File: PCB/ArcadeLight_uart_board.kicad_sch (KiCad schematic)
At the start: 20 parts, among them J1 Partition_Lights_L, J10 Circle_LED, J11 Cross_LED, J12 Square_LED, J13 Triangle_LED, J3 12V_In, J9 Partition_Lights_R, P7 CONN_01X01, P9 CONN_01X01, Q1 AO3404A, Q2 IRFR9024N, U1 Arduino_Nano_v3.x, U2 ULN2003, U3 ULN2003

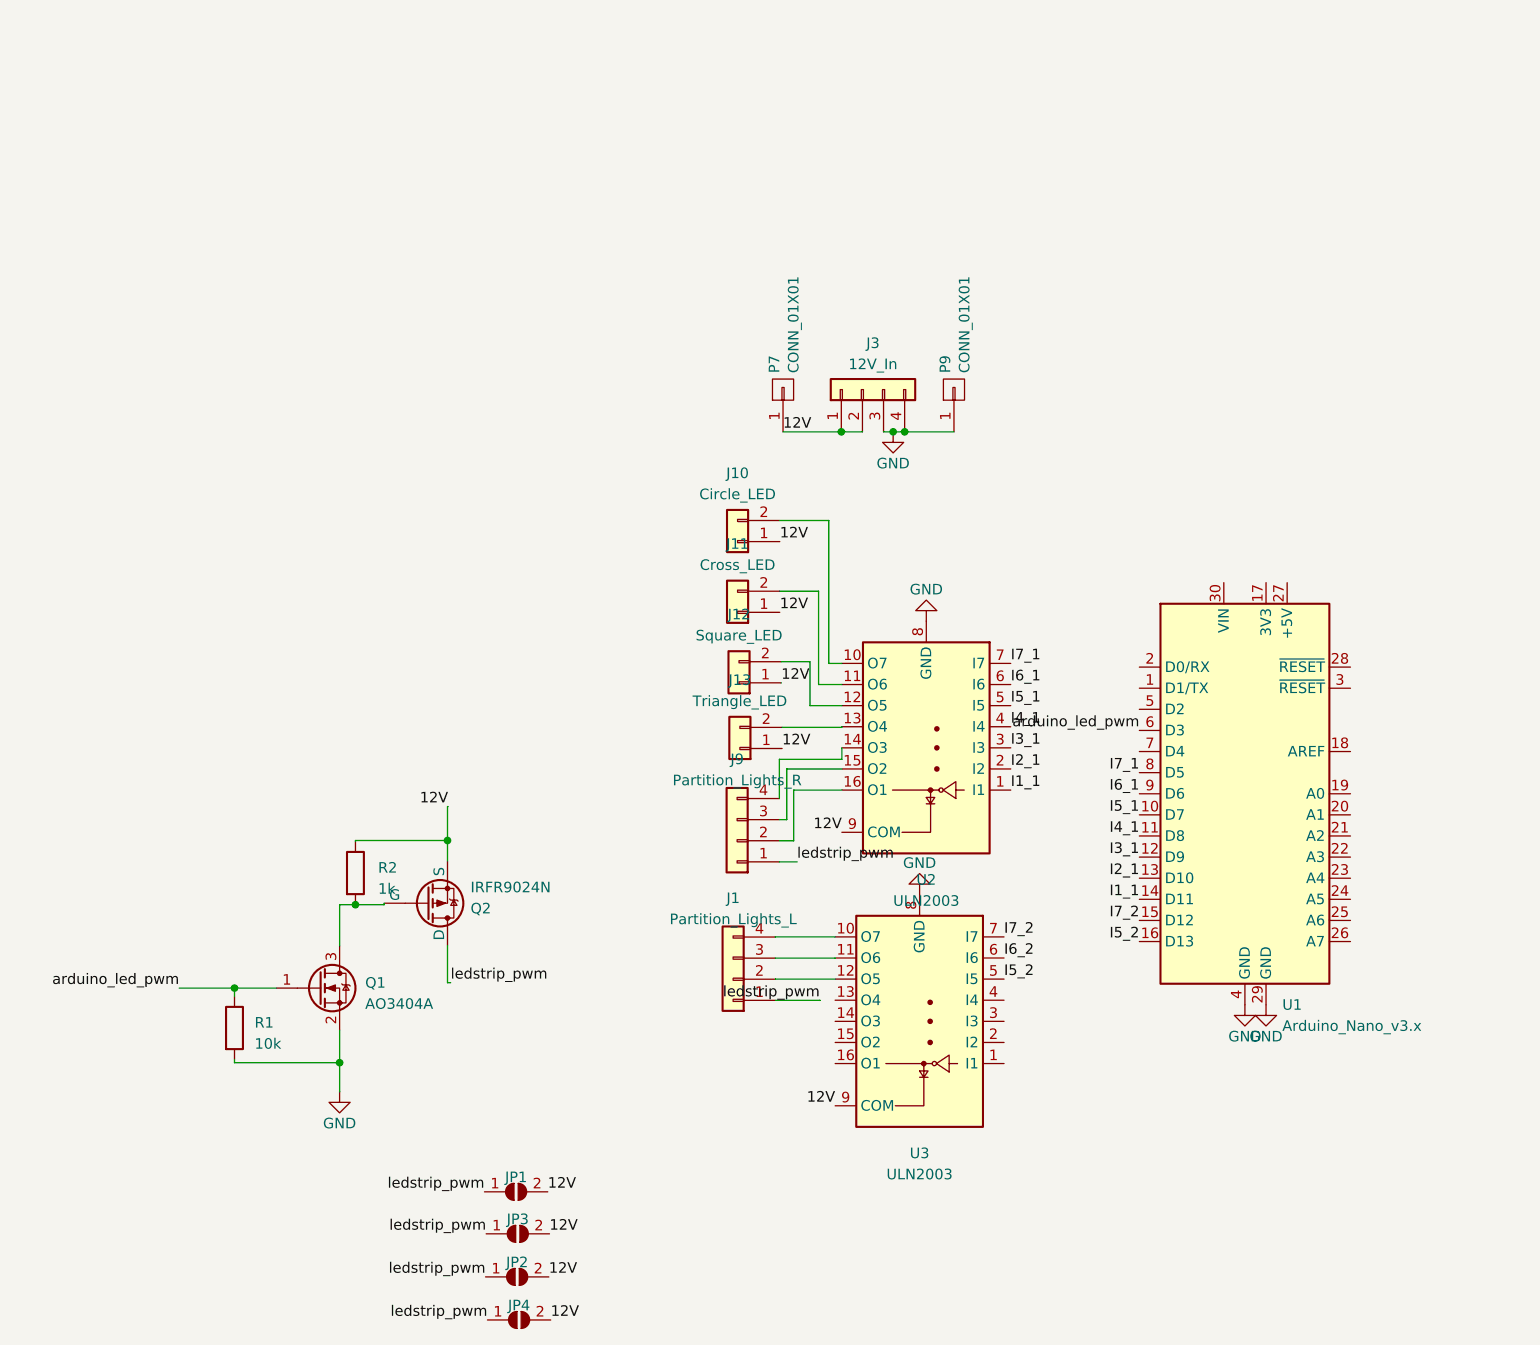
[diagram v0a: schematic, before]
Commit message: Readme update
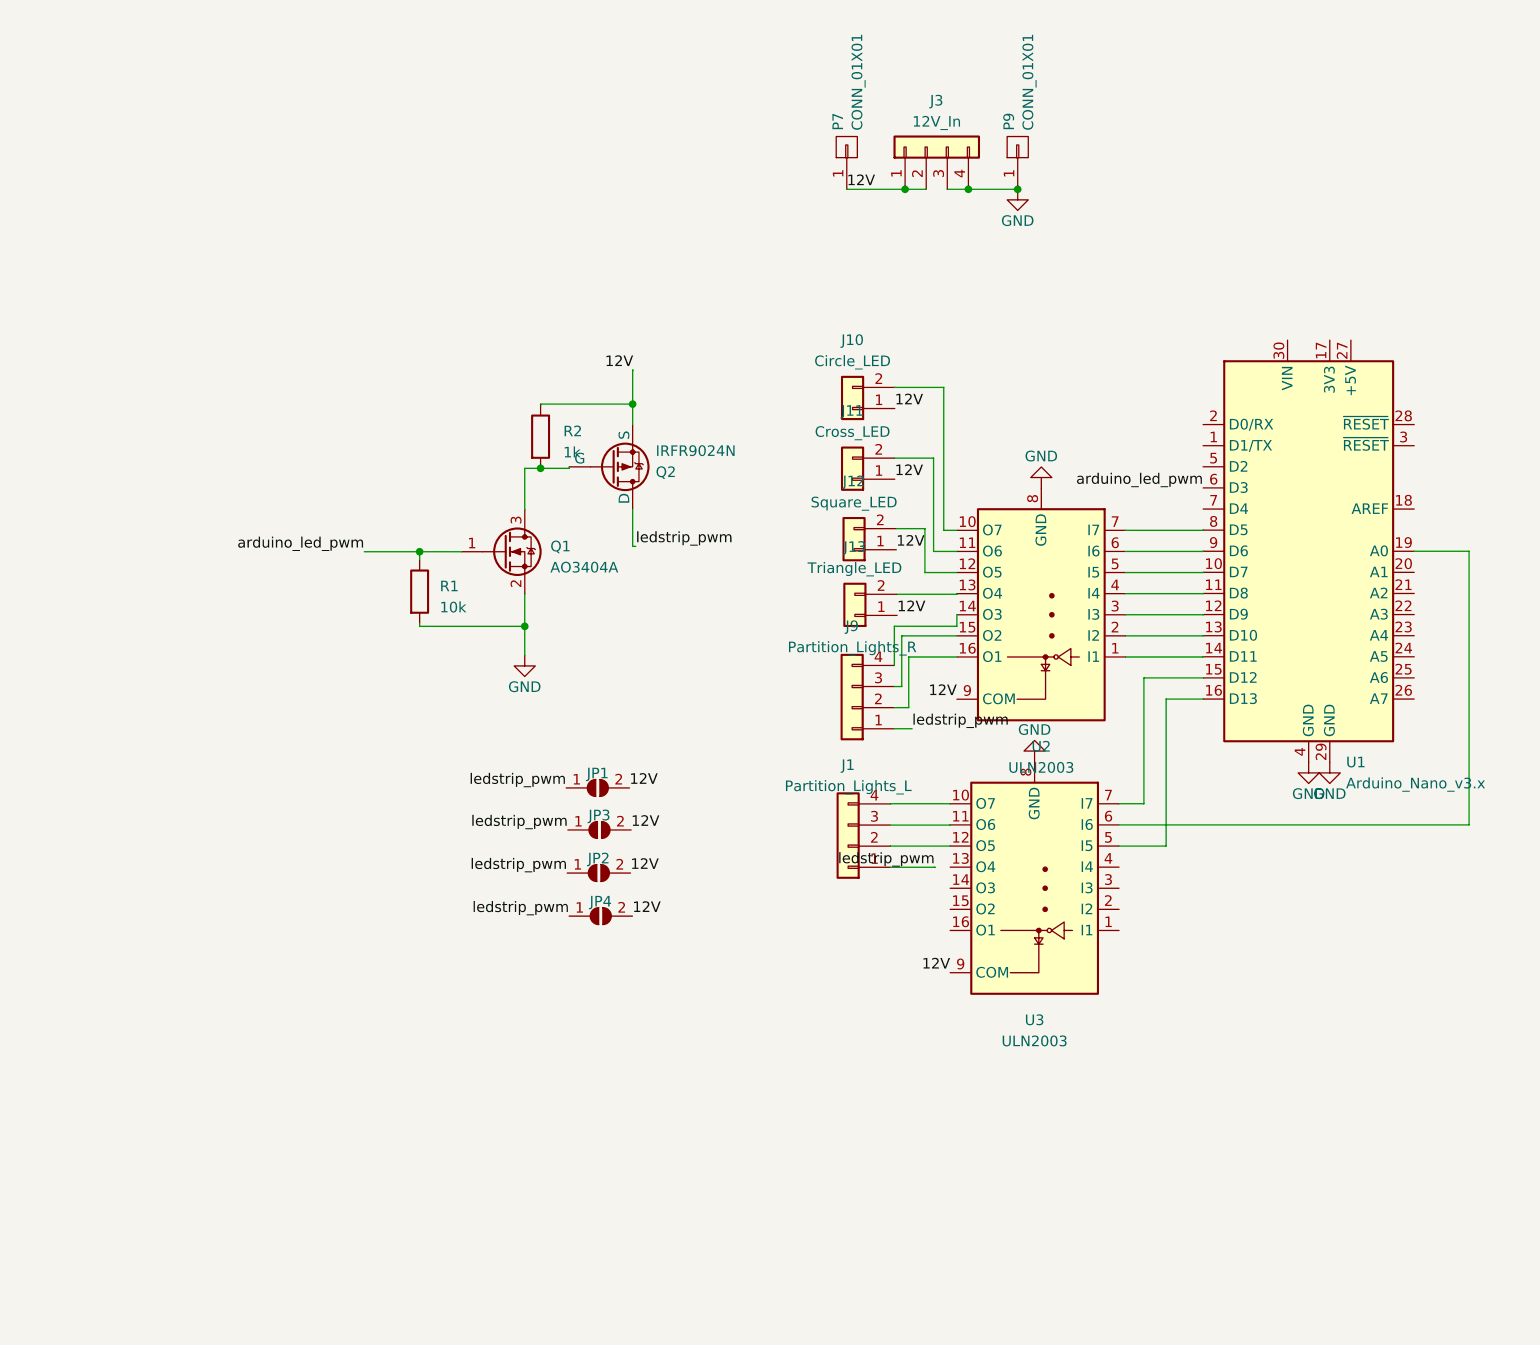
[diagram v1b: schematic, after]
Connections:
- net I6_2 is gone; now on an unnamed net: U3.6 (I6)
- net I1_1: no longer names the net of U1.14 (D11), U2.1 (I1)
- net I2_1: no longer names the net of U1.13 (D10), U2.2 (I2)
- net I3_1: no longer names the net of U1.12 (D9), U2.3 (I3)
- net I4_1: no longer names the net of U1.11 (D8), U2.4 (I4)
- net I5_1: no longer names the net of U1.10 (D7), U2.5 (I5)
- net I5_2: no longer names the net of U1.16 (D13), U3.5 (I5)
- net I6_1: no longer names the net of U1.9 (D6), U2.6 (I6)
- net I7_1: no longer names the net of U1.8 (D5), U2.7 (I7)
- net I7_2: no longer names the net of U1.15 (D12), U3.7 (I7)
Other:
- moved on the sheet: J1, J10, J11, J12, J13, J3, J9, JP1, JP2, JP3, JP4, P7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
